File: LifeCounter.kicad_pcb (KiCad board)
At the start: 2 copper layers, 100.2 x 74.8 mm, 210 parts, among them J201 USBC, J301 Debug, Q201 DO2308S, Q202 DO2309A, Q203 DO2309A, Q601 DO2309A, Q602 DO2309A, Q603 DO2309A, Q604 DO2309A, Q605 DO2309A, Q606 DO2309A, Q607 DO2309A, Q608 DO2309A, Q609 DO2308S, Q610 DO2308S, Q611 DO2308S, Q612 DO2308S, Q701 DO2309A, Q702 DO2309A, Q703 DO2309A, Q704 DO2309A, Q705 DO2309A, Q706 DO2309A, Q707 DO2309A, Q708 DO2309A, Q709 DO2308S, Q710 DO2308S, Q711 DO2308S, Q712 DO2308S, Q801 DO2308S, SW201 PWR_ON, SW301 RST, SW401 RotaryEncoder_Switch_MP, SW501 RotaryEncoder_Switch_MP, U201 TPS630701RNMR, U202 BQ24090DGQ, U203 BQ27441-G1, U301 STM32C031K6Tx, U401 74LVC3G14, U501 74LVC3G14, U601 74HC595, U603 CC56-12GWA, U604 74HC595, U701 74HC595, U703 CC56-12GWA, U704 74HC595

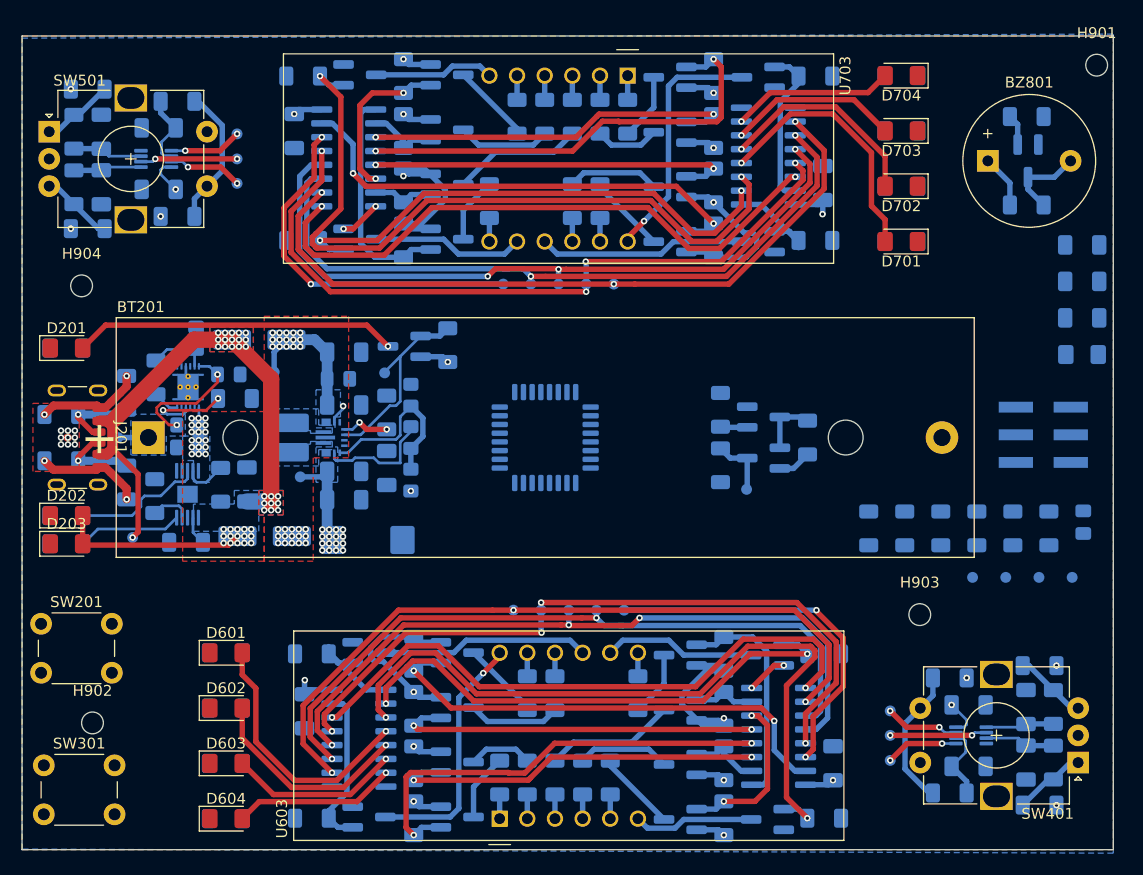
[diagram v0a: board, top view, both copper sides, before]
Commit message: Everything routed :)
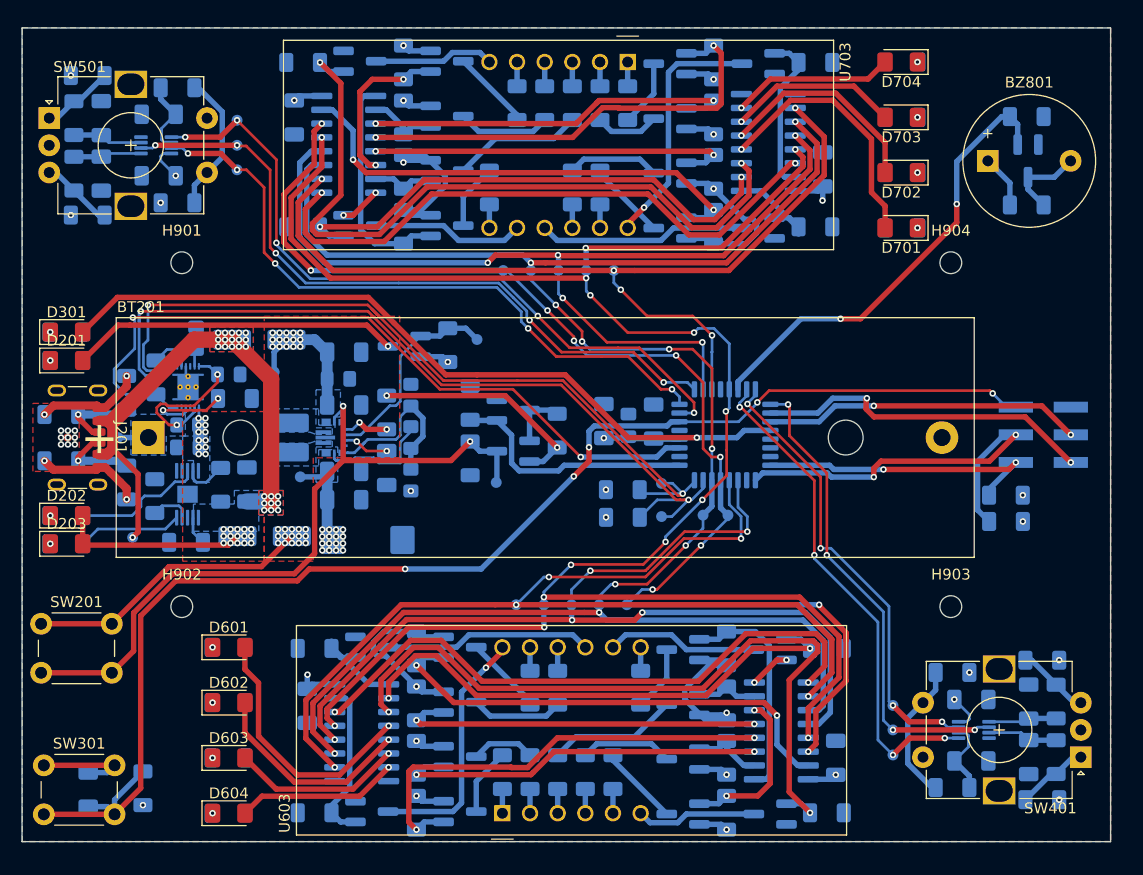
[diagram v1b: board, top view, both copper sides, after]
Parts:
- D301: moved to F.Cu
- moved C301 104.1 mm to (110.1, 121.2), turned to 90 degrees
- moved D301 93.3 mm to (108.1, 79.2), turned to 0 degrees
- moved H901 86.0 mm to (118.7, 72.8)
- moved H904 79.9 mm to (189.3, 72.8)
- moved R302 79.1 mm to (108.1, 79.2), turned to 180 degrees
- moved R301 70.8 mm to (115.1, 121.1)
- moved C302 45.8 mm to (157.4, 87.4), turned to 90 degrees
- moved C303 42.7 mm to (159.7, 87.8), turned to 90 degrees
- moved C304 40.5 mm to (162.0, 87.4), turned to 90 degrees
- moved R304 32.5 mm to (159.2, 96.2), turned to 180 degrees
- moved TP304 32.1 mm to (168.8, 96.0)
- moved TP302 32.1 mm to (162.7, 96.1)
- moved TP303 31.4 mm to (166.6, 96.0)
- moved TP301 29.9 mm to (162.7, 93.1)
- moved R303 29.4 mm to (159.2, 93.7), turned to 180 degrees
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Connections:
- U301 pad 10: /Display1/LAT -> /Display2/LAT
- U301 pad 11: /Display1/~{CLR} -> /Display2/~{CLR}
- U301 pad 15: /Controller/Encoder2.CLK -> /Controller/Encoder1.CLK
- U301 pad 16: /Controller/Encoder2.DAT -> /Controller/Encoder1.DAT
- U301 pad 17: /Controller/Encoder2.BTN -> /Controller/Encoder1.BTN
- U301 pad 27: /Display2/LAT -> /Display1/LAT
- U301 pad 28: /Display2/~{CLR} -> /Display1/~{CLR}
- U301 pad 7: /Controller/Encoder1.CLK -> /Controller/Encoder2.CLK
- U301 pad 8: /Controller/Encoder1.DAT -> /Controller/Encoder2.DAT
- U301 pad 9: /Controller/Encoder1.BTN -> /Controller/Encoder2.BTN
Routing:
- net /Controller/~{RST}: track 0.00 -> 124.7 mm, vias 0 -> 5
- net /Controller/I2C1.SDA: track 0.00 -> 78.3 mm, vias 0 -> 2
- net /Controller/I2C1.SCL: track 0.00 -> 76.0 mm, vias 0 -> 2
- net /Controller/Heartbeat: track 0.00 -> 70.1 mm, vias 0 -> 1
- net /Controller/PWR_OK: track 2.46 -> 69.5 mm, vias 0 -> 2
- net /Controller/Encoder2.CLK: track 6.67 -> 66.3 mm, vias 2 -> 5
- net /Power/EN: track 7.55 -> 66.3 mm, vias 1 -> 2
- net /Controller/Encoder2.BTN: track 8.93 -> 64.7 mm, vias 2 -> 5
- net /Controller/Encoder2.DAT: track 6.86 -> 60.9 mm, vias 2 -> 5
- net /Display1/~{OE}: track 133.5 -> 185.9 mm, vias 8 -> 14
- net /Display1/CLK: track 131.2 -> 180.6 mm, vias 4 -> 10
- net /Display1/DAT: track 68.5 -> 117.9 mm, vias 4 -> 10
- net /Power/VIN: track 15.6 -> 59.6 mm, vias 30 -> 32
- net /Controller/Encoder1.CLK: track 6.67 -> 46.4 mm, vias 2 -> 4
- net /Buzzer/Buzz: track 2.87 -> 41.9 mm, vias 0 -> 2
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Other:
- board size 100.2 x 74.8 mm -> 100 x 74.8 mm
